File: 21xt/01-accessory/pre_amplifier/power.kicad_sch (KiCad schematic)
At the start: 1 part, among them IC1 LT6658AHMSE-5#PBF

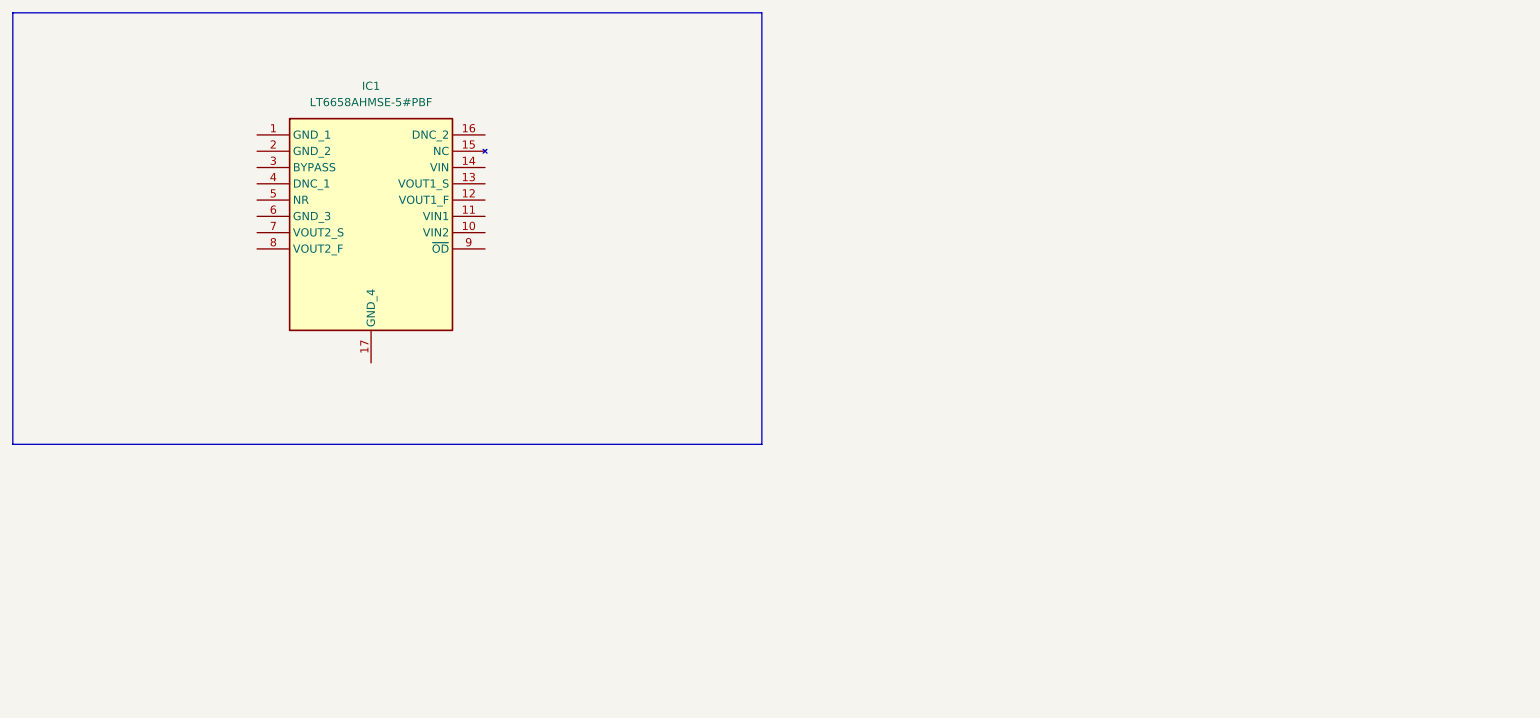
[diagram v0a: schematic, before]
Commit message: Continued schematic
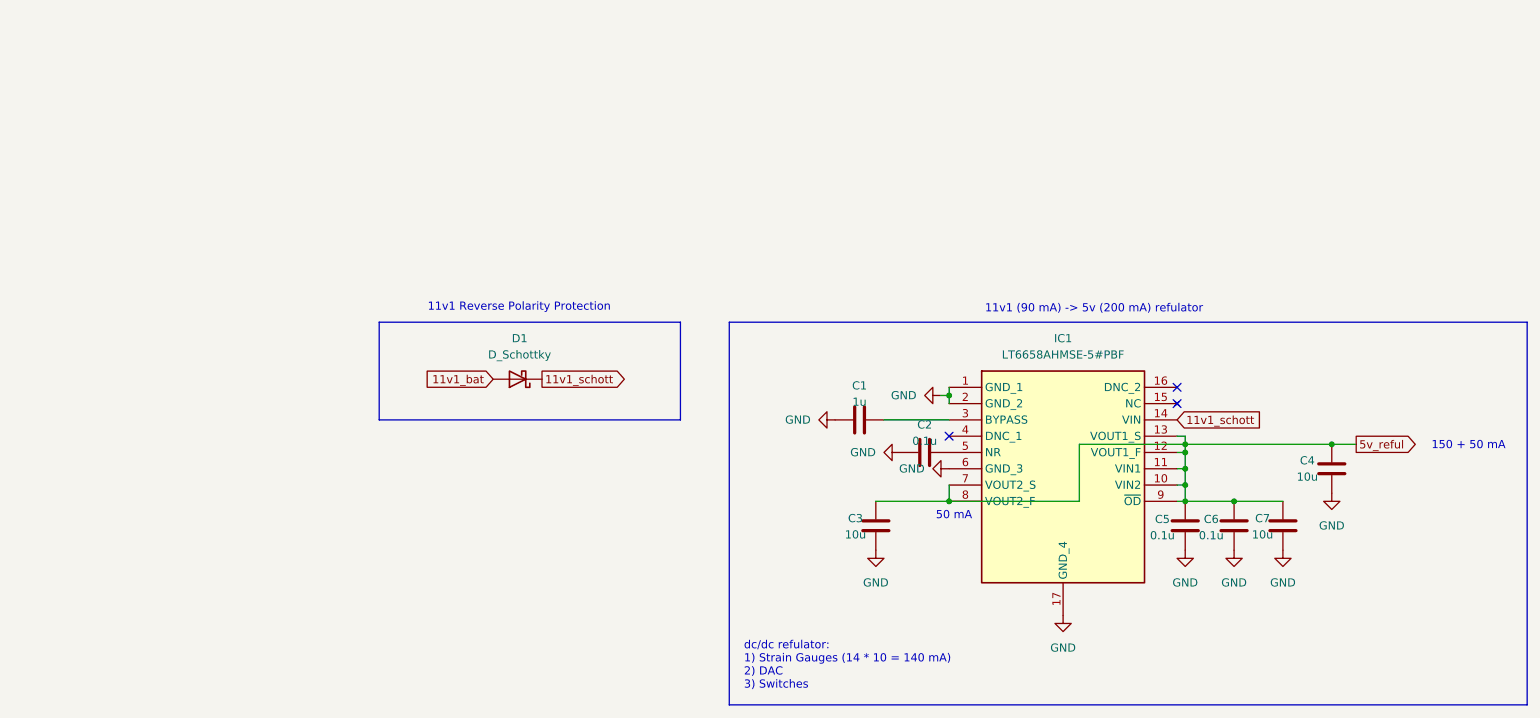
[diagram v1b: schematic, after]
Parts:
- added C1: 1u, symbol Device:C
- added C2, C5, C6: 0.1u, symbol Device:C
- added C3, C4, C7: 10u, symbol Device:C
- added D1: D_Schottky, symbol Device:D_Schottky
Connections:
- net GND: now reaches IC1.1 (GND_1)
- net GND: now also IC1.17 (GND_4), IC1.2 (GND_2), IC1.6 (GND_3), C1.1, C2.1, C3.1, C4.1, C5.1, C6.1, C7.1
- net 5v_reful: now reaches IC1.10 (VIN2)
- net 5v_reful: now also IC1.11 (VIN1), IC1.12 (VOUT1_F), IC1.13 (VOUT1_S), IC1.7 (VOUT2_S), IC1.8 (VOUT2_F), IC1.9 (~{OD}), C3.2, C4.2, C5.2, C6.2, C7.2
- net 11v1_schott: now reaches IC1.14 (VIN)
- net 11v1_schott: now also D1.1 (K)
- net at IC1.3 (BYPASS): now also C1.2
- net at IC1.5 (NR): now also C2.2
- new net 11v1_bat: D1.2 (A)
- no-connect marks 0 -> 3
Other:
- note added: "11v1 (90 mA) -> 5v (200 mA) refulator"
- note added: "11v1 Reverse Polarity Protection"
- note added: "150 + 50 mA"
- note added: "50 mA"
- note added: "dc/dc refulator: 1) Strain Gauges (14 * 10 = 140 mA) 2) DAC 3) Switches"
- moved on the sheet: IC1
